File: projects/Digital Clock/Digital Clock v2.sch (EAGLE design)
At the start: 29 parts, among them U1 FT232RL-BASICSSOP

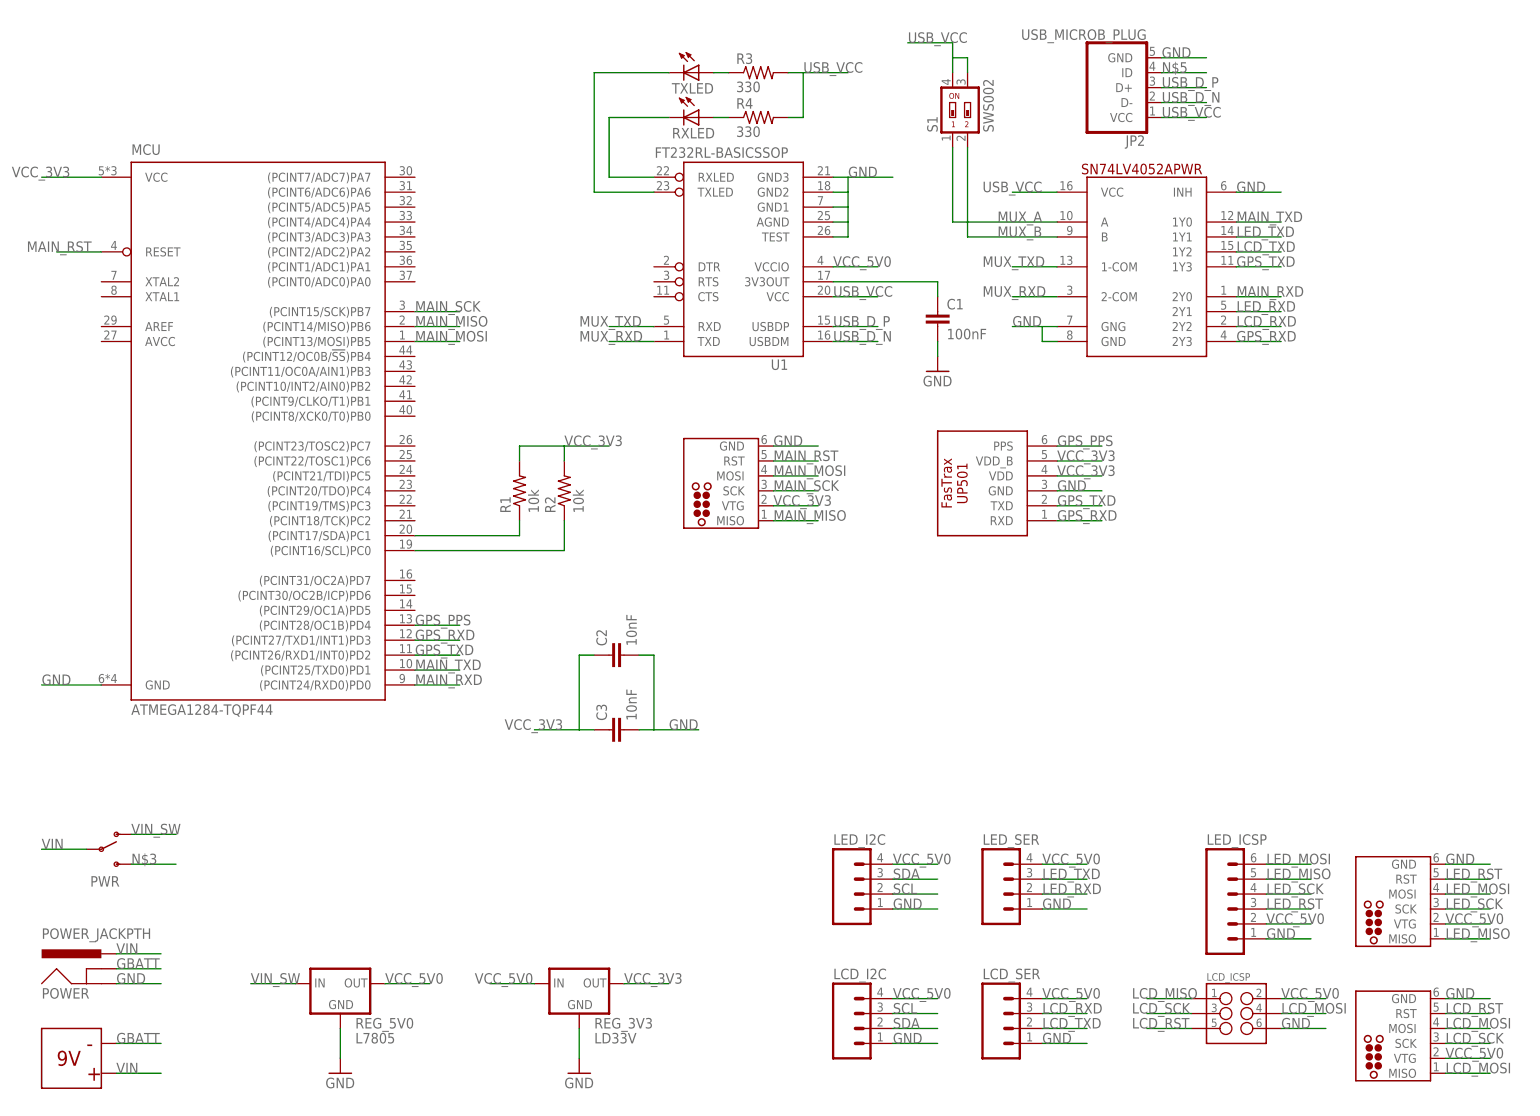
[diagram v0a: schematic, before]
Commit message: Many minor revisions to Digital Clock v2
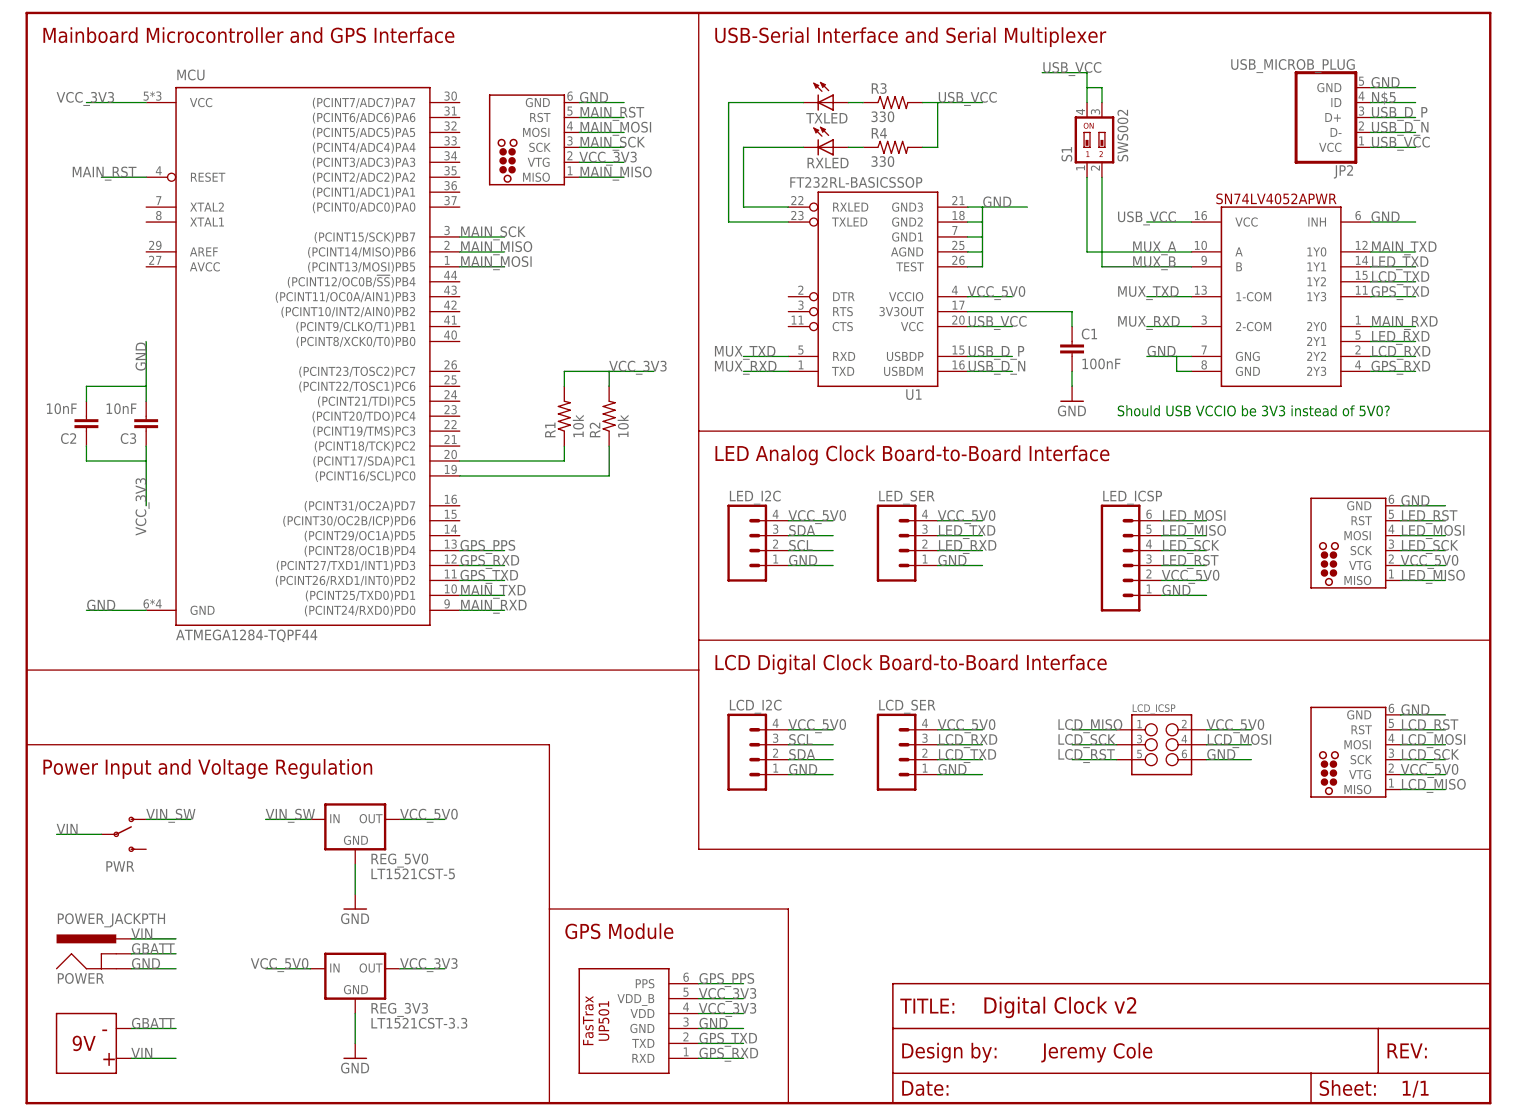
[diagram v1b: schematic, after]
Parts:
- added FRAME1: FRAME-LETTERNO_PACKAGE, jcole:FRAME-LETTERNO_PACKAGE
- REG_3V3: value LD33V -> LT1521CST-3.3; device SparkFun:V_REG_78XXSIDE -> jcole:LT1521
- REG_5V0: value L7805 -> LT1521CST-5; device SparkFun:V_REG_78XXSIDE -> jcole:LT1521
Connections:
- removed net N$3: PWR.S
- net LCD_MISO: now also LCD_ICSP_TC.MISO
- net LCD_MOSI: no longer LCD_ICSP_TC.MISO
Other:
- note added: "GPS Module"
- note added: "Jeremy Cole"
- note added: "LCD Digital Clock Board-to-Board Interface"
- note added: "LED Analog Clock Board-to-Board Interface"
- note added: "Mainboard Microcontroller and GPS Interface"
- note added: "Power Input and Voltage Regulation"
- note added: "Should USB VCCIO be 3V3 instead of 5V0?"
- note added: "USB-Serial Interface and Serial Multiplexer"
- moved on the sheet: C1, C2, C3, JP2, LCD_I2C, LCD_ICSP, LCD_SER, LED_I2C, LED_ICSP, LED_SER, MCU, POWER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
